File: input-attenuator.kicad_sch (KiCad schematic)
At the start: 71 parts, among them J1 DC_INTF, J2 RF_IN, J3 RX_1_RF, J4 RX_2_RF, K1 EE2-5TNU-L, K2 EE2-5TNU-L, K3 EE2-5TNU-L, K4 EE2-5TNU-L, Q1 BC858, Q2 BC858, Q3 MMBT3904, Q4 BC858, Q5 BC858, Q6 BC858, Q7 BC858, Q8 BC858, Q9 BC858, U1 74HC00, U2 74HC00, U3 74HC00, U4 74HC00, U5 74HC00, U6 74HC595

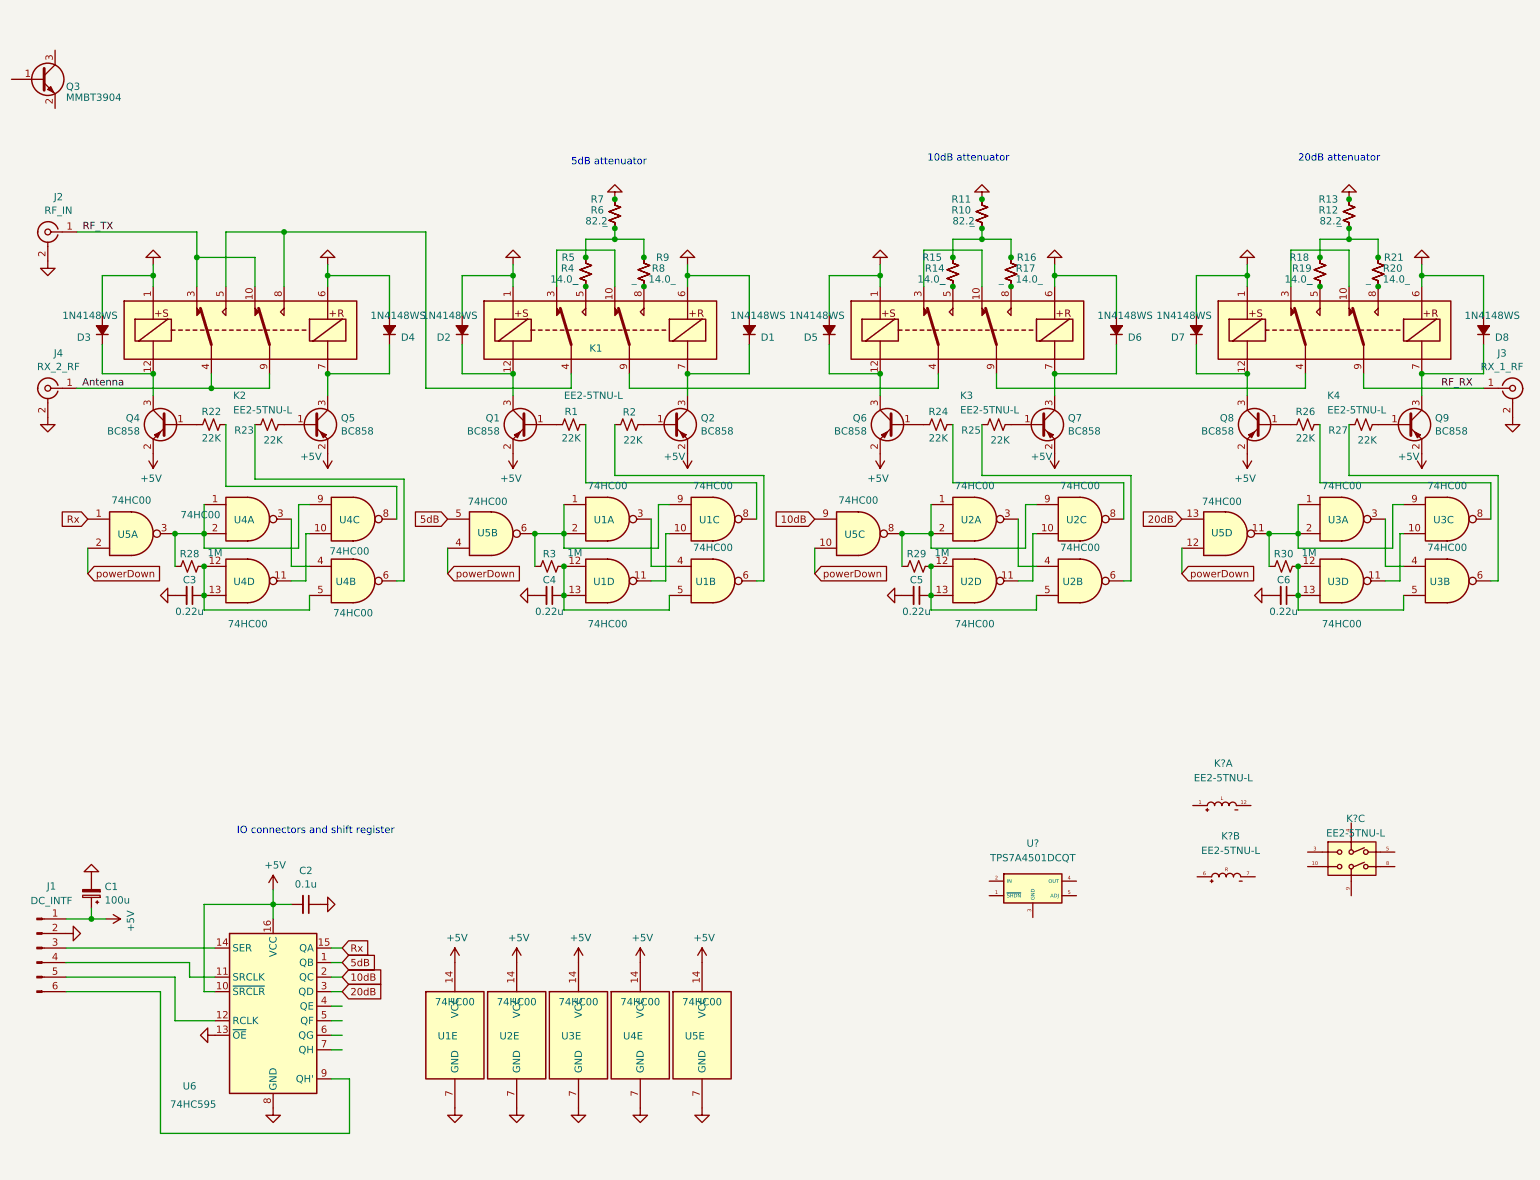
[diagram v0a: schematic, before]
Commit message: addedPowerDown
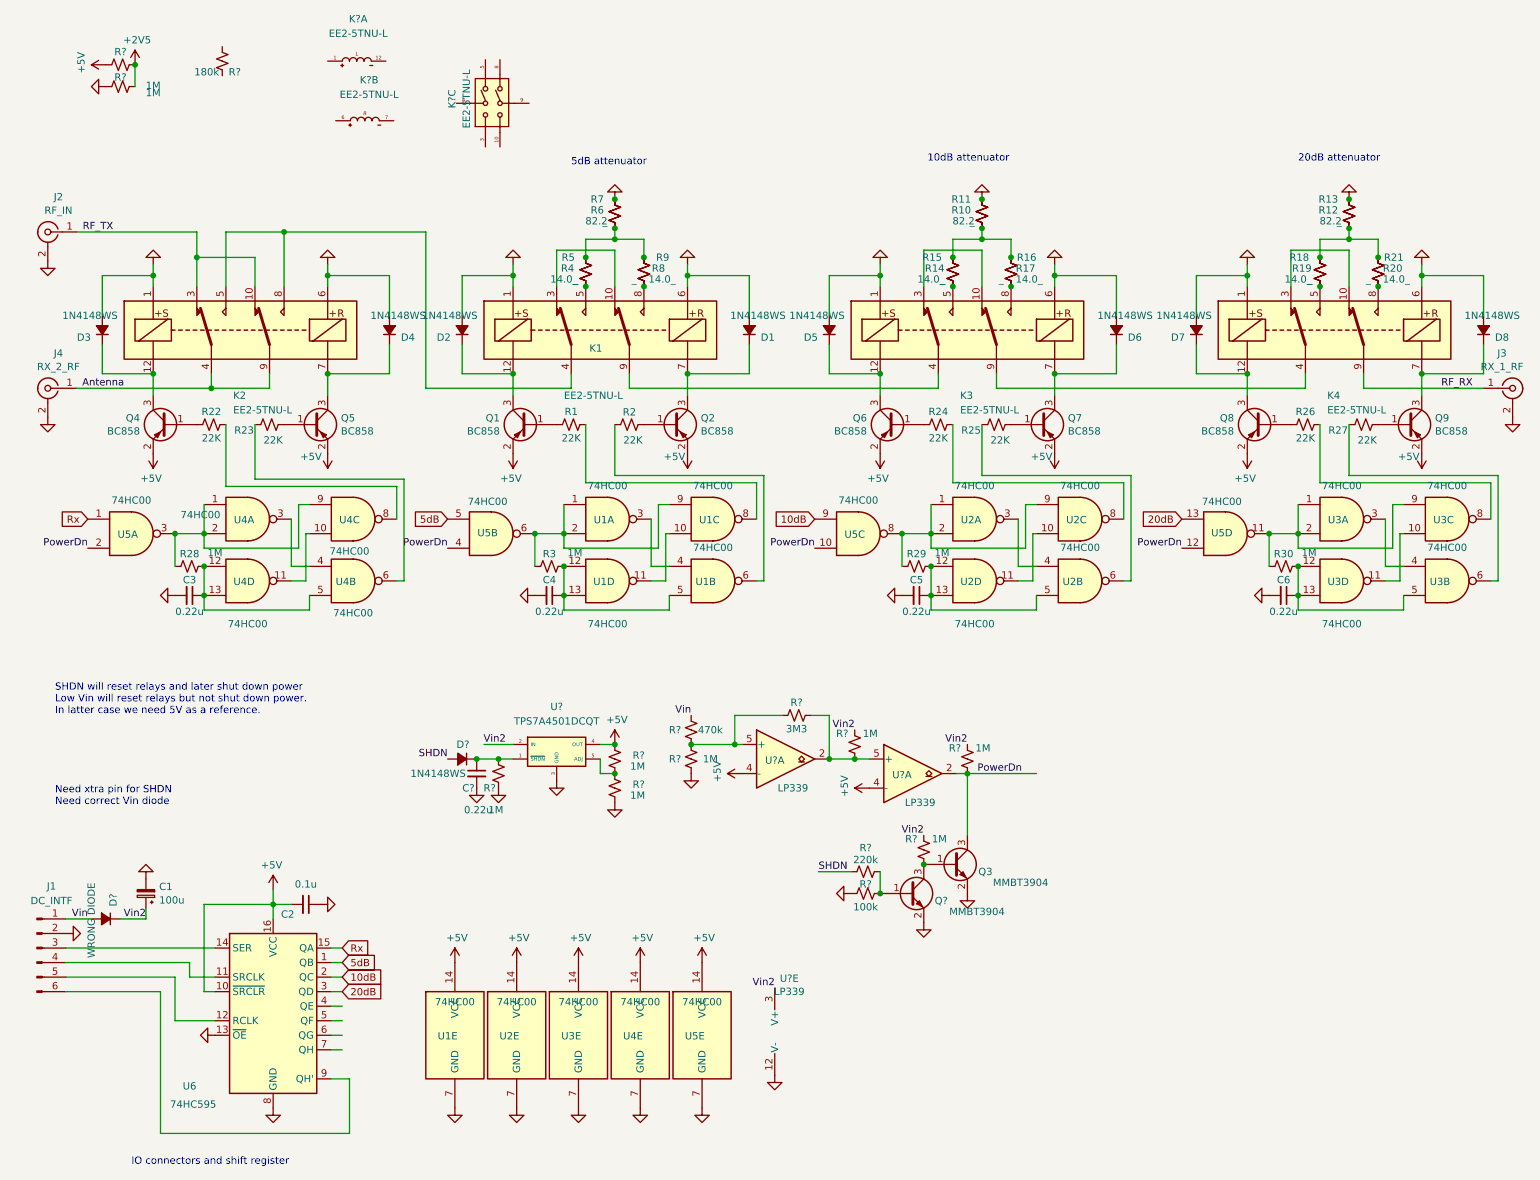
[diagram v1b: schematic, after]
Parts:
- added C?: 0.22u, Capacitor_SMD:C_0805_2012Metric, symbol Device:C_Small
- added D?: 1N4148WS, Diode_SMD:D_SOD-323, symbol Device:D_Small_ALT
- added D?: WRONG DIODE, Diode_SMD:D_SOD-323, symbol Device:D_Small_ALT
- added Q?: MMBT3904, Package_TO_SOT_SMD:SOT-23, symbol Transistor_BJT:MMBT3904
- added R?: 180k, Resistor_SMD:R_0805_2012Metric, symbol Device:R_Small_US
- added R? (x9): 1M, Resistor_SMD:R_0805_2012Metric, symbol Device:R_Small_US
- added R?: 220k, Resistor_SMD:R_0805_2012Metric, symbol Device:R_Small_US
- added R?: 3M3, Resistor_SMD:R_0805_2012Metric, symbol Device:R_Small_US
- added R?: 470k, Resistor_SMD:R_0805_2012Metric, symbol Device:R_Small_US
- added R?: 100k, Resistor_SMD:R_0805_2012Metric, symbol Device:R_Small_US
- added U? (x3): LP339, symbol Comparator:LM339
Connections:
- net powerDown is gone; now on net PowerDn: U5.10, U5.12, U5.2, U5.4
- net +5V: now also U?.4 (OUT), R?.2, R?.2, U?.4 (-), U?.4 (-); no longer C1.1, J1.1 (Pin_1)
- net GND: now also Q3.2 (E), U?.3 (GND), C?.2, Q?.2 (E), R?.1, R?.1, R?.1, R?.2, R?.2, U?.12 (V-)
- net at Q3.1 (B): now also Q?.3 (C), R?.1
- net PowerDn: now reaches Q3.3 (C)
- net PowerDn: now also R?.1, U?.2
- net at U?.1 (~SHDN): now also C?.1, D?.1 (K), R?.2
- net Vin2: now reaches U?.2 (IN)
- net Vin2: now also C1.1, D?.1 (K), R?.2, R?.2, R?.2, U?.3 (V+)
- net at U?.5 (ADJ): now also R?.1, R?.2
- new net: R?.1, R?.1, U?.2, U?.5 (+)
- new net: Q?.1 (B), R?.1, R?.1
- new net: R?.1, R?.2, R?.2, U?.5 (+)
- new net +2V5: R?.1, R?.1
- new net SHDN: D?.2 (A), R?.2
- new net Vin: D?.2 (A), J1.1 (Pin_1), R?.2
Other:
- note added: "Need xtra pin for SHDN Need correct Vin diode"
- note added: "SHDN will reset relays and later shut down power Low Vin will reset relays but not shut down power. In latter case we need 5V as a reference."
- moved on the sheet: C1, K?A, K?B, K?C, Q3, U?
